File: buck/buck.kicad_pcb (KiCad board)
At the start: 2 copper layers, 19.5 x 8.5 mm, 14 parts, among them J1 Conn_01x02_Male, J2 Conn_01x02_Male, U1 TPMP2359DJ

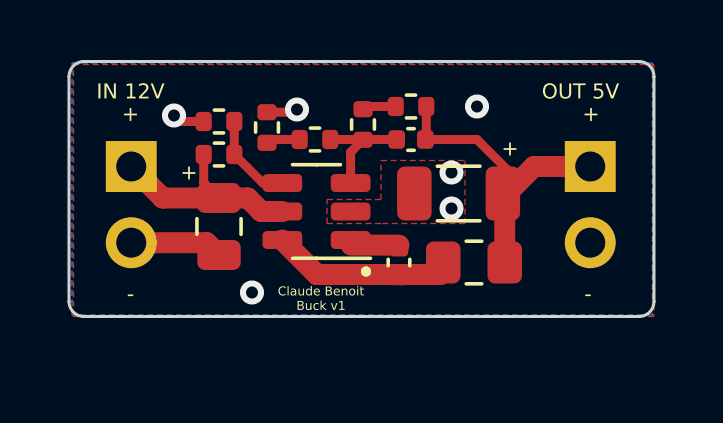
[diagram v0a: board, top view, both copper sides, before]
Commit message: update for JLCPCB
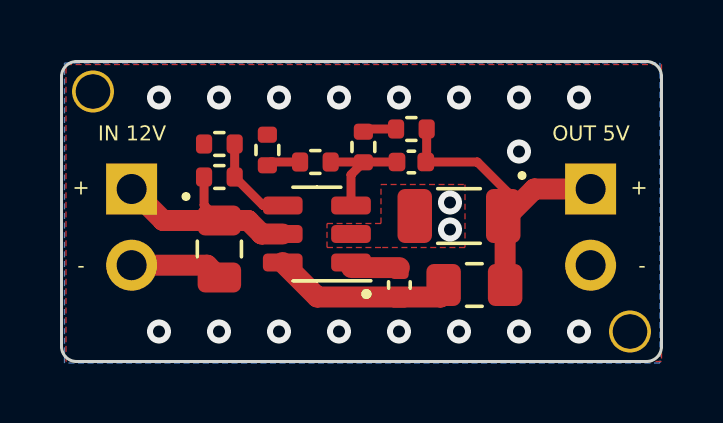
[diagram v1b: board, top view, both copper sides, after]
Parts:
- added REF**: JLCPCB Tooling Hole, Library:JLCPCB Tooling Hole, F.Cu at (86.4, 68.8)
- added REF**: JLCPCB Tooling Hole, Library:JLCPCB Tooling Hole, F.Cu at (68.5, 60.8)
- moved C1 0.75 mm to (72.7, 66.0)
- moved C2 0.75 mm to (78.7, 67.2)
- moved C3 0.75 mm to (80.7, 64.9)
- moved C4 0.75 mm to (79.1, 63.1)
- moved J2 0.75 mm to (85.1, 64.0)
- moved L1 0.75 mm to (81.2, 67.2)
- moved R1 0.75 mm to (72.7, 63.6)
- moved R2 0.75 mm to (72.7, 62.5)
- moved R3 0.75 mm to (79.1, 62.0)
- moved R5 0.75 mm to (74.3, 62.7)
- moved R6 0.75 mm to (77.5, 62.6)
- moved U1 0.75 mm to (76.0, 65.5)
- moved J1 0.75 mm to (69.8, 64.0)
- moved R4 0.75 mm to (75.9, 63.1)
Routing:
- net GND: track 5.20 -> 3.09 mm, vias 6 -> 19
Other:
- board size 19.5 x 8.5 mm -> 20 x 10 mm
- board text added: "JLCPCB Tooling Hole"
